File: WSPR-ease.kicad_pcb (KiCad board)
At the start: 4 copper layers, 100 x 75 mm, 106 parts, among them J1 GNSS Ant, J2 Tx Ant, J3 USB_C_16P_Stacked, Q1 MMBF170, Q10 MMBF170, Q11 MMBF170, Q12 MMBF170, Q13 MMBF170, Q2 MMBF170, Q3 MMBF170, Q4 MMBF170, Q5 MMBF170, Q6 MMBF170, Q7 MMBF170, Q8 MMBF170, Q9 MMBF170, T1 BN-43-202_DualPri_CTSec, U1 ESP32-S3-WROOM-1, U2 NCP1117-3.3_SOT223, U3 ATGM336H-5N31, U4 ICE40UP5K-SG48ITR, U5 TLV70012, U6 CD74ACT541M96G4

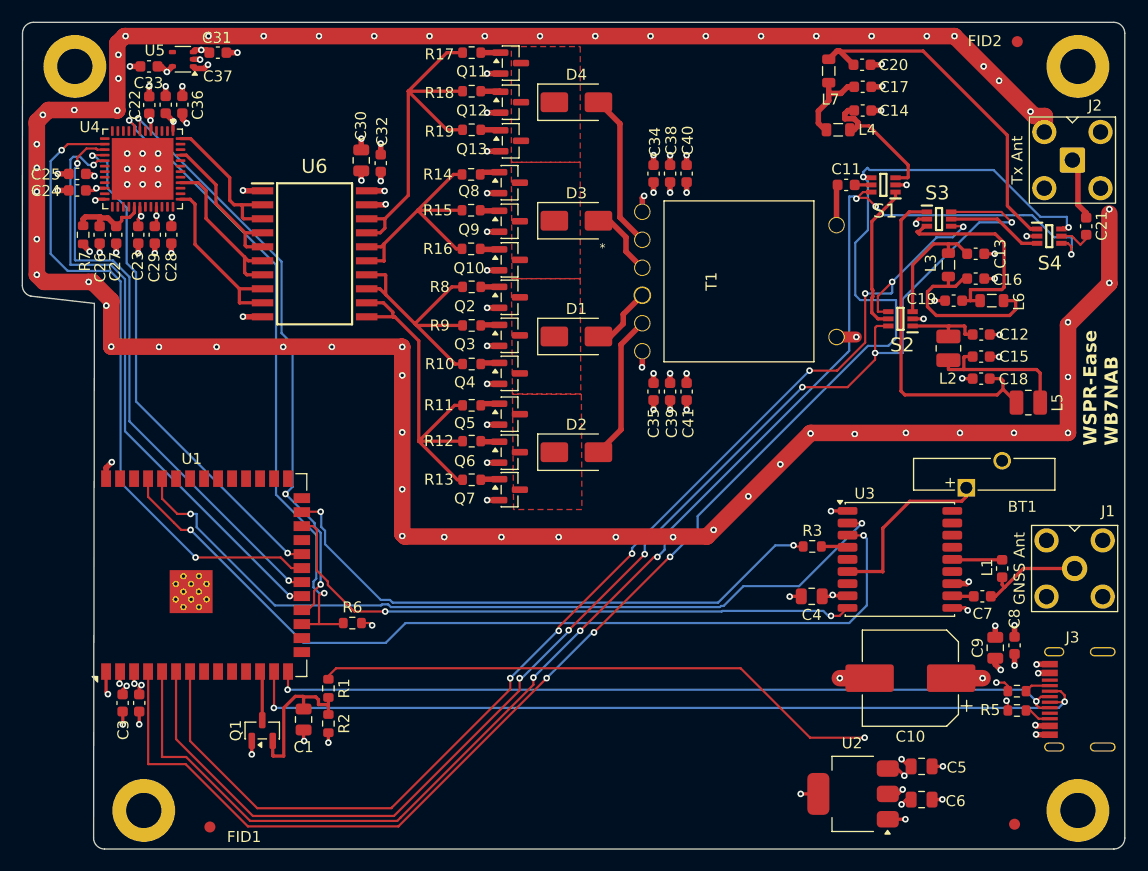
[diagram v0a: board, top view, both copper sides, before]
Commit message: Minor tweaks after submitting 001 build to pcbway
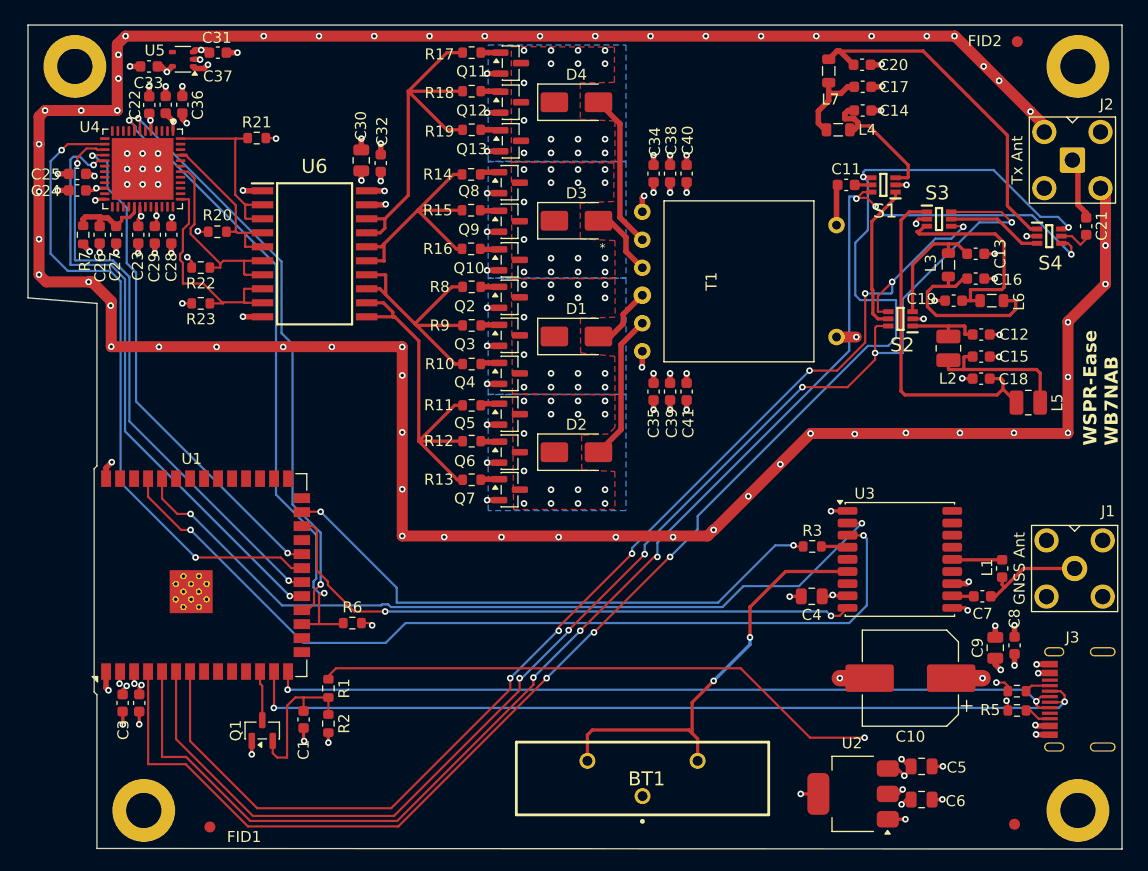
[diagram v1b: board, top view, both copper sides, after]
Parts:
- added R20: 10k, Resistor_SMD:R_0603_1608Metric, F.Cu at (67.3, 77.4)
- added R21: 10k, Resistor_SMD:R_0603_1608Metric, F.Cu at (70.8, 68.9)
- added R22: 10k, Resistor_SMD:R_0603_1608Metric, F.Cu at (65.8, 80.7)
- added R23: 10k, Resistor_SMD:R_0603_1608Metric, F.Cu at (65.8, 83.9)
- BT1: value CR1220 -> S8401-46; footprint Battery:Battery_Panasonic_CR1220-VCN_Vertical_CircularHoles -> Library:S8401-46
- C1: footprint Capacitor_SMD:C_0805_2012Metric -> Capacitor_SMD:C_0603_1608Metric
- moved BT1 39.5 mm to (105.8, 127.0), turned to 180 degrees
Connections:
- net Net-(D1-A) renamed /Transmitter/push1T
- net Net-(D2-A) renamed /Transmitter/push2T
- net Net-(D3-A) renamed /Transmitter/pull1T
- net Net-(D4-A) renamed /Transmitter/pull2T
- BT1 pad 1: Net-(BT1-+) -> GND
- BT1 pad 2: GND -> Net-(U3-V_BCKP)
- D3 pad 1: /Transmitter/pull2D -> /Transmitter/pull1D
- D4 pad 1: /Transmitter/pull1D -> /Transmitter/pull2D
- Q10 pad 3: /Transmitter/pull2D -> /Transmitter/pull1D
- Q11 pad 3: /Transmitter/pull1D -> /Transmitter/pull2D
- Q12 pad 3: /Transmitter/pull1D -> /Transmitter/pull2D
- Q13 pad 3: /Transmitter/pull1D -> /Transmitter/pull2D
- Q8 pad 3: /Transmitter/pull2D -> /Transmitter/pull1D
- Q9 pad 3: /Transmitter/pull2D -> /Transmitter/pull1D
- U3 pad 6: Net-(BT1-+) -> Net-(U3-V_BCKP)
- U4 pad 40: /Transmitter/push1 -> unconnected-(U4A-RGB1-Pad40)
- U4 pad 42: unconnected-(U4A-IOT_51a-Pad42) -> /Transmitter/push1
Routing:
- net Net-(U3-V_BCKP): track 0.00 -> 38.7 mm, vias 0 -> 2
- net Net-(BT1-+): track 16.7 -> 0.00 mm
- net GND: track 338.3 -> 343.5 mm, vias 139 -> 141
- net /Transmitter/push2: track 16.3 -> 21.0 mm
- net /Transmitter/push1: track 15.0 -> 18.6 mm
- net /Transmitter/pull2: track 14.2 -> 16.9 mm
- net /Transmitter/pull1: track 14.1 -> 16.0 mm
- net /loON: track 132.1 -> 131.0 mm
- net /hiON: track 139.9 -> 139.1 mm
- net /fpgaDONE: track 54.4 -> 53.7 mm, vias 3 -> 2
- net /gnssTx: track 74.6 -> 73.9 mm
- net Net-(U1-IO48): track 52.6 -> 51.9 mm
- net /Transmitter/pull2D: track 0.00 -> 0.07 mm, vias 0 -> 16
- net /Transmitter/pull1D: track 0.07 -> 0.00 mm, vias 0 -> 16
- net /Transmitter/push2D: vias 0 -> 16
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- added copper zone on B.Cu, net /Transmitter/pull1D
- added copper zone on B.Cu, net /Transmitter/pull2D
- added copper zone on B.Cu, net /Transmitter/push1D
- added copper zone on B.Cu, net /Transmitter/push2D
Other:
- board size 100 x 75 mm -> 99.2 x 74.8 mm
